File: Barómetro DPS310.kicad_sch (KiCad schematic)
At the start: 0 parts

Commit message: Protocolos I2C/SPI
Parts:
- added C24, C25: 100nF, easyeda2kicad:C0402, symbol CANSAT_STM32_symbols:TCC0402X7R104J500AT
- added R1: 100k, symbol Device:R
- added R4, R5: 4.7K, easyeda2kicad:R0603, symbol CANSAT_STM32_symbols:RC0603FR-074K7L
- added U5: DPS310XTSA1, easyeda2kicad:LGA-8_DPS310XTSA1, symbol CANSAT_STM32_symbols:DPS310XTSA1
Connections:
- new net +3.3V: C25.2, R4.2, R5.2, U5.6 (VDDIO)
- new net +3.3VA: C24.1, U5.8 (VDD)
- new net DPS_INT: R1.1, U5.5 (SDO)
- new net GND: C24.2, C25.1, R1.2, U5.1 (GND), U5.7 (GND)
- new net I2C1_SCL: R5.1, U5.4 (SCK)
- new net I2C1_SDA: R4.1, U5.3 (SDI)
- no-connect marks 0 -> 1

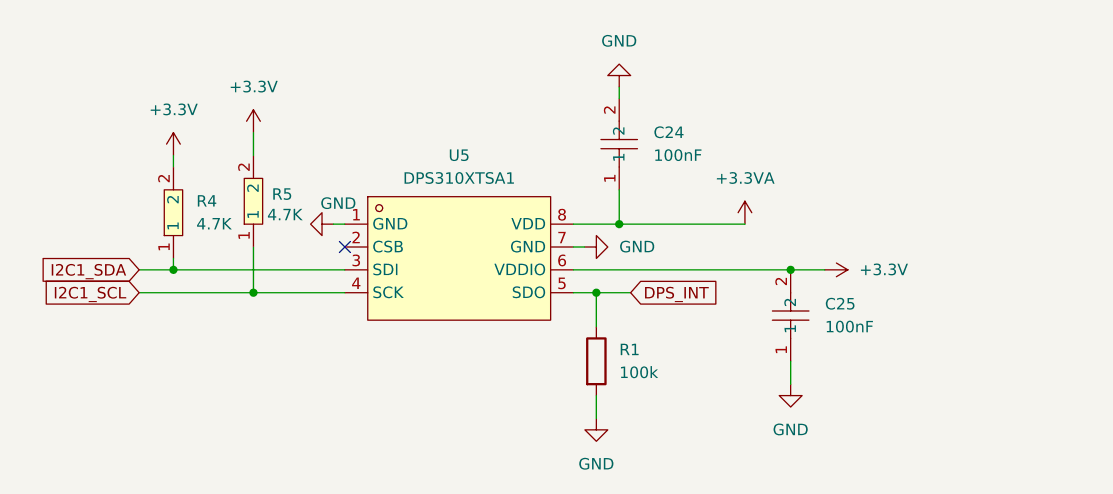
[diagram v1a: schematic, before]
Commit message: BECERRA
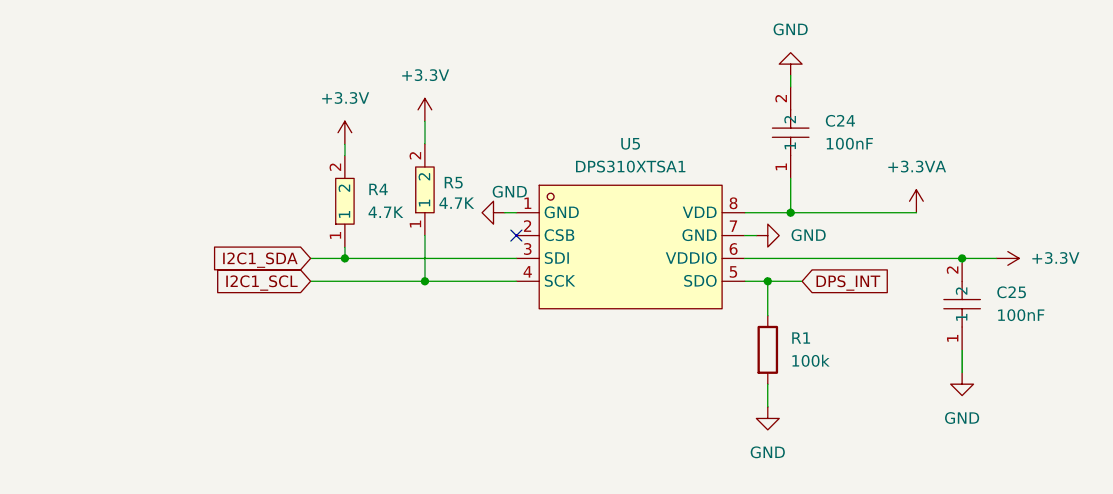
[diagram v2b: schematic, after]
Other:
- moved on the sheet: C24, C25, R1, R4, R5, U5
